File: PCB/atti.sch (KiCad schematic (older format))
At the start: 35 parts, among them J1 Conn_02x04_Counter_Clockwise, J2 FTSH-105-01-X-D-007-K, J3 Conn_01x01_Female, J5 Conn_01x01_Female, J6 Conn_01x01_Female, J7 Conn_01x01_Female, SW1 SW_SPST, U1 AP2112K-3.3, U2 STM32F303K8Tx, U3 NVT2006, U5 BMX160, U6 BMP280, Y1 32 MHz

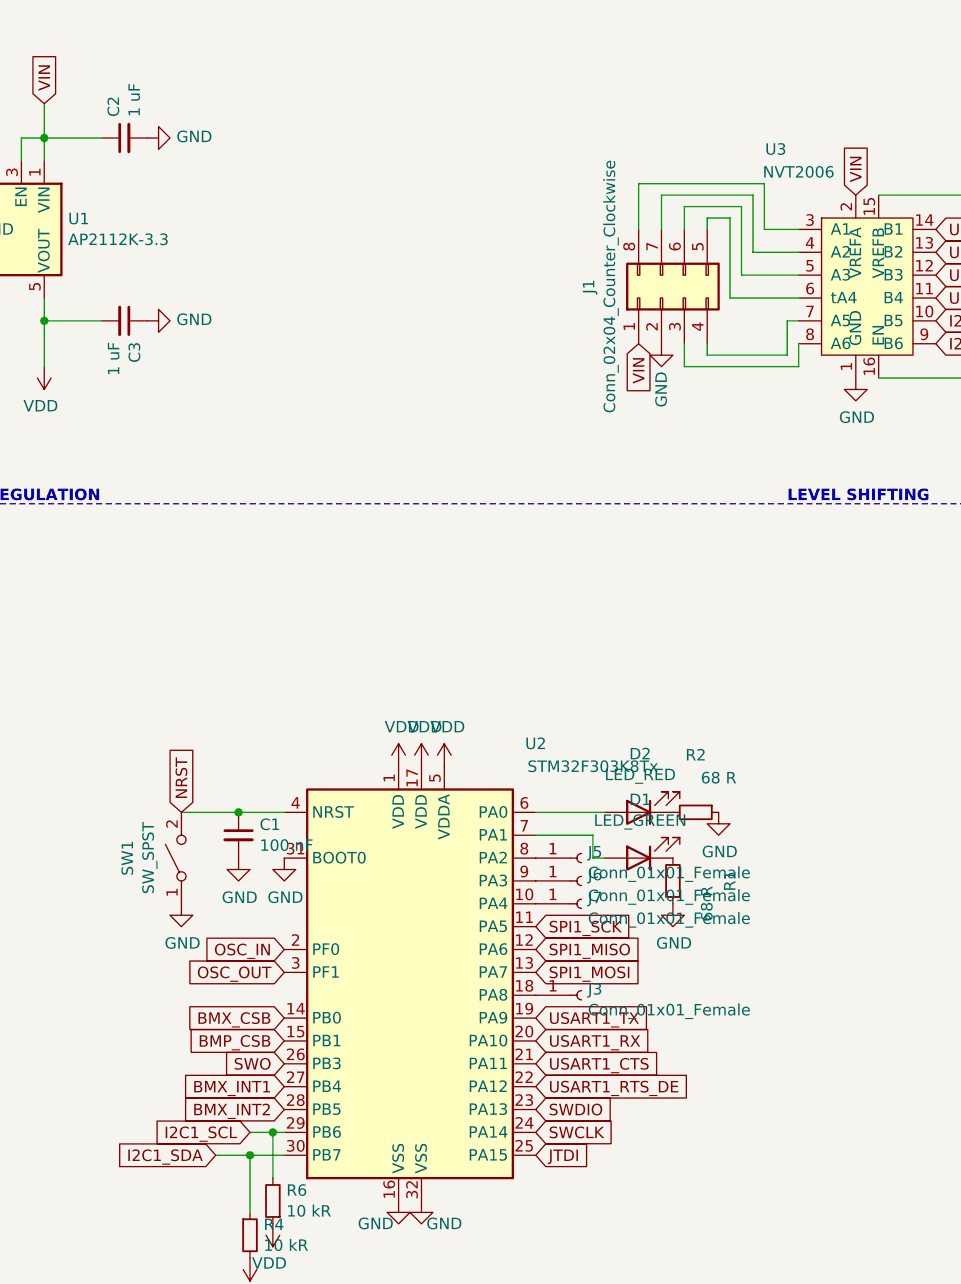
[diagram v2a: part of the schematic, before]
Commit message: Good routing progress
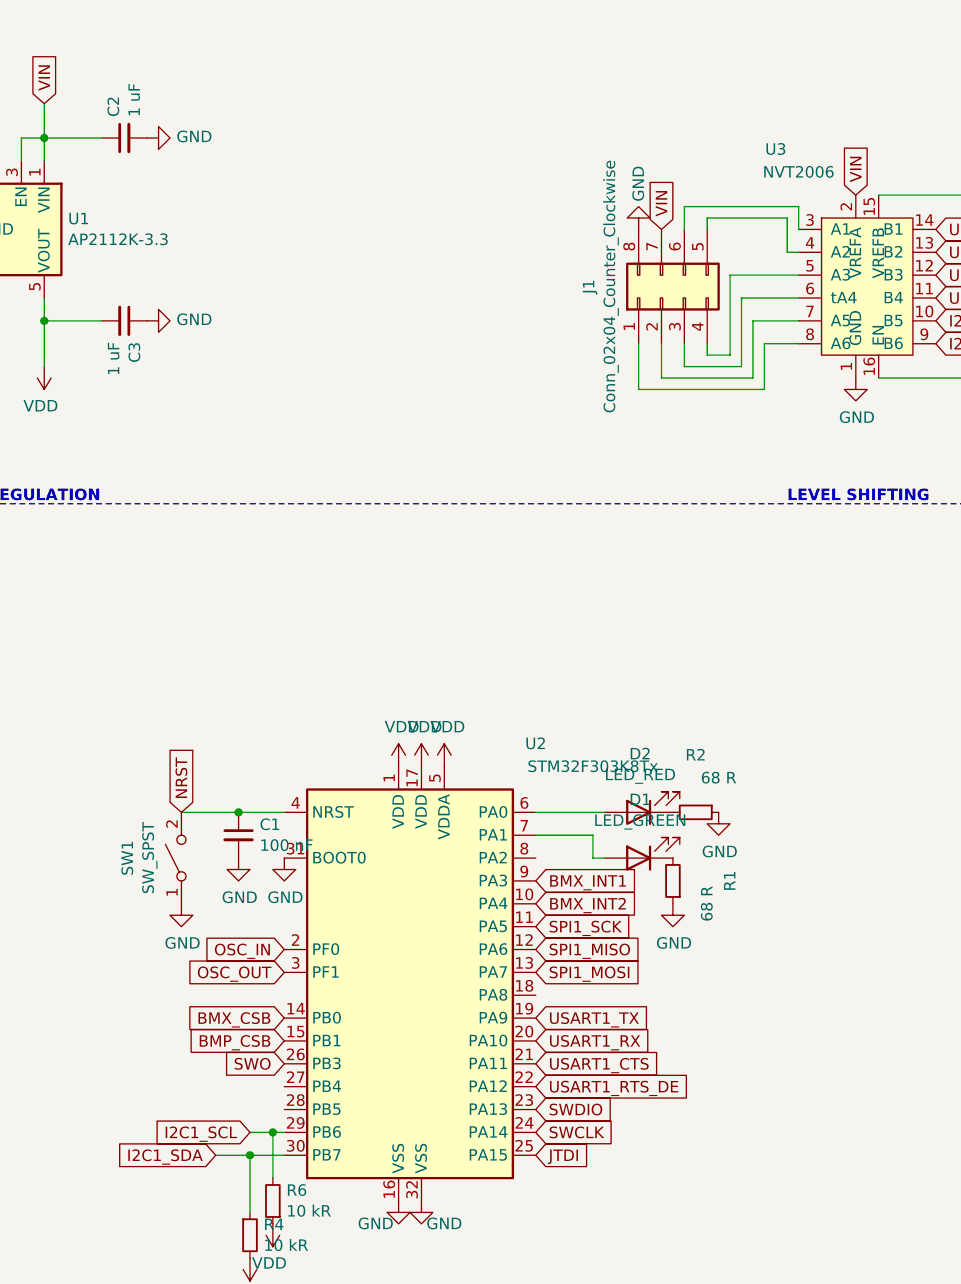
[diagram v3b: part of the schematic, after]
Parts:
- removed J3, J5, J6, J7: Conn_01x01_Female, Connector_Wire:SolderWire-0.25sqmm_1x01_D0.65mm_OD1.7mm, symbol Connector:Conn_01x01_Female
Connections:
- net BMX_INT1: now also U2.9 (PA3); no longer U2.27 (PB4)
- net BMX_INT2: now also U2.10 (PA4); no longer U2.28 (PB5)
- net GND: now also J1.8 (Pin_8); no longer J1.2 (Pin_2)
- net VIN: now also J1.7 (Pin_7); no longer J1.1 (Pin_1)
- net at U3.8 (A6): now also J1.1 (Pin_1); no longer J1.3 (Pin_3)
- net at U3.7 (A5): now also J1.2 (Pin_2); no longer J1.4 (Pin_4)
- net at U3.6 (tA4): now also J1.3 (Pin_3); no longer J1.5 (Pin_5)
- net at U3.5 (A3): now also J1.4 (Pin_4); no longer J1.6 (Pin_6)
- net at U3.4 (A2): now also J1.5 (Pin_5); no longer J1.7 (Pin_7)
- net at U3.3 (A1): now also J1.6 (Pin_6); no longer J1.8 (Pin_8)
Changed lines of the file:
@@
 Text GLabel 5650 1400 2    50   Input ~ 0
 USART1_TX
-Text GLabel 4350 1900 3    50   Input ~ 0
+Text GLabel 4450 1400 1    50   Input ~ 0
 VIN
 $Comp
 L power:GND #PWR?
 U 1 1 5FDAC75D
-P 4450 1900
-F 0 "#PWR?" H 4450 1650 50  0001 C CNN
-F 1 "GND" V 4450 1700 50  0000 C CNN
-F 2 "" H 4450 1900 50  0001 C CNN
-F 3 "" H 4450 1900 50  0001 C CNN
-	1    4450 1900
-	1    0    0    -1
+P 4350 1400
+F 0 "#PWR?" H 4350 1150 50  0001 C CNN
+F 1 "GND" V 4350 1200 50  0000 C CNN
+F 2 "" H 4350 1400 50  0001 C CNN
+F 3 "" H 4350 1400 50  0001 C CNN
+	1    4350 1400
+	-1   0    0    1
 $EndComp
 Wire Wire Line
@@
 Text GLabel 10650 1550 2    50   Input ~ 0
 BMX_INT2
-Text GLabel 2800 5150 0    50   Input ~ 0
+Text GLabel 3900 4250 2    50   Input ~ 0
 BMX_INT1
 $Comp
@@
 	-1   0    0    1
 $EndComp
-$Comp
-L Connector:Conn_01x01_Female J7
-U 1 1 5FDFE414
-P 4100 4350
-F 0 "J7" H 4128 4376 50  0000 L CNN
-F 1 "Conn_01x01_Female" H 4128 4285 50  0000 L CNN
-F 2 "Connector_Wire:SolderWire-0.25sqmm_1x01_D0.65mm_OD1.7mm" H 4100 4350 50  0001 C CNN
-F 3 "~" H 4100 4350 50  0001 C CNN
-	1    4100 4350
-	1    0    0    -1
-$EndComp
-$Comp
-L Connector:Conn_01x01_Female J5
-U 1 1 5FDFF854
-P 4100 4150
-F 0 "J5" H 4128 4176 50  0000 L CNN
-F 1 "Conn_01x01_Female" H 4128 4085 50  0000 L CNN
-F 2 "Connector_Wire:SolderWire-0.25sqmm_1x01_D0.65mm_OD1.7mm" H 4100 4150 50  0001 C CNN
-F 3 "~" H 4100 4150 50  0001 C CNN
-	1    4100 4150
-	1    0    0    -1
-$EndComp
-$Comp
-L Connector:Conn_01x01_Female J6
-U 1 1 5FE016CD
-P 4100 4250
-F 0 "J6" H 4128 4276 50  0000 L CNN
-F 1 "Conn_01x01_Female" H 4128 4185 50  0000 L CNN
-F 2 "Connector_Wire:SolderWire-0.25sqmm_1x01_D0.65mm_OD1.7mm" H 4100 4250 50  0001 C CNN
-F 3 "~" H 4100 4250 50  0001 C CNN
-	1    4100 4250
-	1    0    0    -1
-$EndComp
 Wire Wire Line
 	4150 4150 4200 4150
 Wire Wire Line
 	3900 4050 4150 4050
-$Comp
-L Connector:Conn_01x01_Female J3
-U 1 1 5FE09C11
-P 4100 4750
-F 0 "J3" H 4128 4776 50  0000 L CNN
-F 1 "Conn_01x01_Female" H 4128 4685 50  0000 L CNN
-F 2 "Connector_Wire:SolderWire-0.25sqmm_1x01_D0.65mm_OD1.7mm" H 4100 4750 50  0001 C CNN
-F 3 "~" H 4100 4750 50  0001 C CNN
-	1    4100 4750
-	1    0    0    -1
-$EndComp
 $Comp
 L Device:Crystal_GND24_Small Y1
@@
 	0    -1   -1   0
 $EndComp
-Text GLabel 2800 5250 0    50   Input ~ 0
+Text GLabel 3900 4350 2    50   Input ~ 0
 BMX_INT2
 Text GLabel 3900 5250 2    50   Input ~ 0
@@
 Text Notes 9150 4500 0    50   ~ 10
 DEBUG
+Text GLabel 2800 5050 0    50   Input ~ 0
+SWO
+Text GLabel 1750 850  1    50   Input ~ 0
+VIN
 $Comp
 L Connector_Generic:Conn_02x04_Counter_Clockwise J1
@@
 $EndComp
 Wire Wire Line
-	5050 1900 5050 2000
-Wire Wire Line
-	5050 2000 4550 2000
+	5050 1300 4550 1300
+Wire Wire Line
+	4550 1300 4550 1400
+Wire Wire Line
+	5050 1300 5050 1400
+Wire Wire Line
+	5050 1500 5000 1500
+Wire Wire Line
+	5000 1500 5000 1350
+Wire Wire Line
+	5000 1350 4650 1350
+Wire Wire Line
+	4650 1350 4650 1400
+Wire Wire Line
+	5050 1600 4750 1600
+Wire Wire Line
+	4750 1600 4750 1950
+Wire Wire Line
+	4750 1950 4650 1950
+Wire Wire Line
+	4650 1950 4650 1900
+Wire Wire Line
+	5050 1700 4800 1700
+Wire Wire Line
+	4800 1700 4800 2000
+Wire Wire Line
+	4800 2000 4550 2000
 Wire Wire Line
 	4550 2000 4550 1900
 Wire Wire Line
-	5050 1800 5000 1800
-Wire Wire Line
-	5000 1800 5000 1950
-Wire Wire Line
-	5000 1950 4650 1950
-Wire Wire Line
-	4650 1950 4650 1900
-Wire Wire Line
-	5050 1700 4750 1700
-Wire Wire Line
-	4750 1700 4750 1350
-Wire Wire Line
-	4750 1350 4650 1350
-Wire Wire Line
-	4650 1350 4650 1400
-Wire Wire Line
-	5050 1600 4800 1600
-Wire Wire Line
-	4800 1600 4800 1300
-Wire Wire Line
-	4800 1300 4550 1300
-Wire Wire Line
-	4550 1300 4550 1400
-Wire Wire Line
-	5050 1500 4850 1500
-Wire Wire Line
-	4850 1500 4850 1250
-Wire Wire Line
-	4850 1250 4450 1250
-Wire Wire Line
-	4450 1250 4450 1400
-Wire Wire Line
-	5050 1400 4900 1400
-Wire Wire Line
-	4900 1400 4900 1200
-Wire Wire Line
-	4900 1200 4350 1200
-Wire Wire Line
-	4350 1200 4350 1400
-Text GLabel 2800 5050 0    50   Input ~ 0
-SWO
-Text GLabel 1750 850  1    50   Input ~ 0
-VIN
+	5050 1800 4850 1800
+Wire Wire Line
+	4850 1800 4850 2050
+Wire Wire Line
+	4850 2050 4450 2050
+Wire Wire Line
+	4450 2050 4450 1900
+Wire Wire Line
+	5050 1900 4900 1900
+Wire Wire Line
+	4900 1900 4900 2100
+Wire Wire Line
+	4900 2100 4350 2100
+Wire Wire Line
+	4350 2100 4350 1900
 $EndSCHEMATC
